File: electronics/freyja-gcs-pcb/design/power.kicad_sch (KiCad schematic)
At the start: 122 parts, among them J6 GT-USB-7010ASV, J7 A2543WR-4P-2, J8 XD-PH-10AW, J9 JS350-S02DCA-00, Q1 TM10N06SI, Q2 TM10N06SI, Q3 AO4459, Q4 L2N7002SLLT1G, Q5 L2N7002SLLT1G, Q6 TM10N06SI, Q7 TM10N06SI, Q8 TM10N06SI, SW3 K6-6136D-L1-04, U10 LM74700QDBVRQ1, U11 AMS1117-3.3, U12 RY3730, U3 FM7021DB, U4 CN3702, U5 HY2213-BB3A, U6 HY2213-BB3A, U7 IP2721, U8 SY8368AQQC, U9 LM74700QDBVRQ1

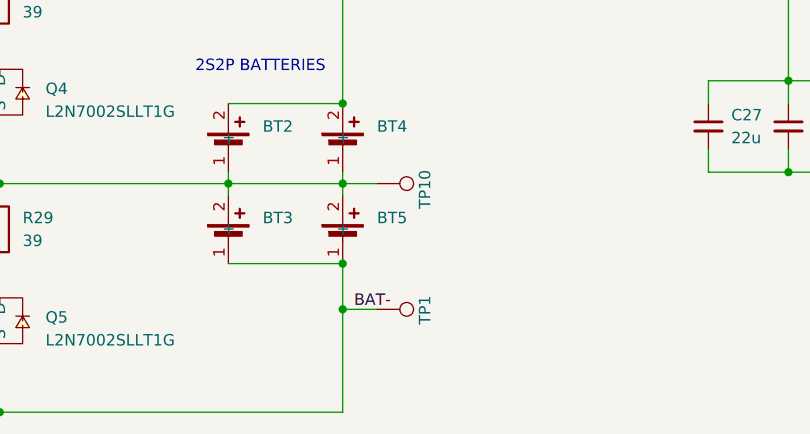
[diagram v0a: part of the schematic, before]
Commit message: cleanup
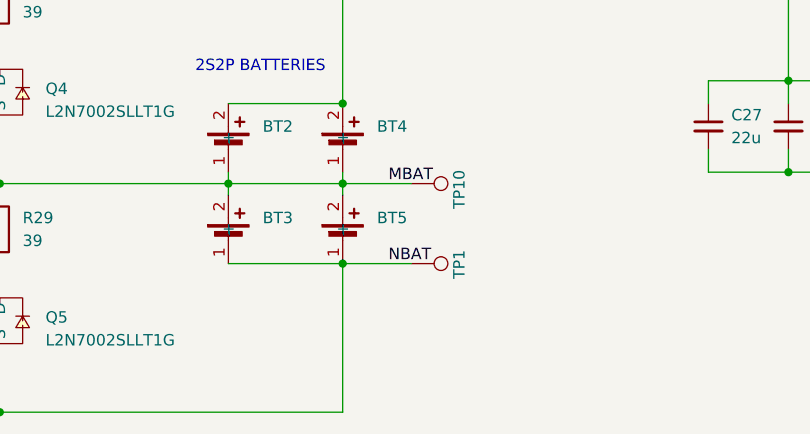
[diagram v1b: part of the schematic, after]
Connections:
- net MBAT: now reaches BT2.1 (-), BT3.2 (+), BT4.1 (-), BT5.2 (+), C21.2, Q4.2 (S), R22.2, R24.1, R29.1, TP10.1, U5.3 (VSS)
- net BAT- renamed NBAT
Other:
- moved on the sheet: TP1, TP10
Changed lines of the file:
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@@
 	)
 	(junction
-		(at 170.18 246.38)
-		(diameter 0)
-		(color 0 0 0 0)
-	)
-	(junction
 		(at 303.53 146.05)
 		(diameter 0)
@@
 	(wire
 		(pts
-			(xy 170.18 246.38) (xy 170.18 257.81)
-		)
-		(stroke
-			(width 0)
-			(type default)
-		)
-	)
-	(wire
-		(pts
 			(xy 274.32 175.26) (xy 276.86 175.26)
 		)
@@
 	(wire
 		(pts
-			(xy 170.18 241.3) (xy 170.18 246.38)
-		)
-		(stroke
-			(width 0)
-			(type default)
-		)
-	)
-	(wire
-		(pts
 			(xy 148.59 44.45) (xy 148.59 49.53)
 		)
@@
 	(wire
 		(pts
+			(xy 170.18 241.3) (xy 170.18 257.81)
+		)
+		(stroke
+			(width 0)
+			(type default)
+		)
+	)
+	(wire
+		(pts
 			(xy 85.09 132.08) (xy 85.09 134.62)
 		)
@@
 	(wire
 		(pts
-			(xy 170.18 246.38) (xy 173.99 246.38)
+			(xy 170.18 241.3) (xy 177.8 241.3)
 		)
 		(stroke
@@
 	(wire
 		(pts
-			(xy 170.18 232.41) (xy 173.99 232.41)
+			(xy 170.18 232.41) (xy 177.8 232.41)
 		)
 		(stroke
@@
 		)
 	)
-	(label "BAT-"
-		(at 171.45 246.38 0)
+	(label "NBAT"
+		(at 175.26 241.3 0)
+		(effects
+			(font
+				(size 1.27 1.27)
+			)
+			(justify left bottom)
+		)
+	)
+	(label "MBAT"
+		(at 175.26 232.41 0)
 		(effects
 			(font
@@
 	(symbol
 		(lib_id "Connector:TestPoint")
-		(at 173.99 232.41 270)
+		(at 177.8 232.41 270)
 		(unit 1)
 		(exclude_from_sim no)
@@
 		(dnp no)
 		(property "Reference" "TP10"
-			(at 179.324 230.886 0)
+			(at 183.134 230.886 0)
 			(effects
 				(font
@@
 		)
 		(property "Value" "TestPoint"
-			(at 176.0221 234.95 0)
+			(at 179.8321 234.95 0)
 			(effects
 				(font
@@
 		)
 		(property "Footprint" "TestPoint:TestPoint_Pad_D3.0mm"
-			(at 173.99 237.49 0)
+			(at 177.8 237.49 0)
 			(effects
 				(font
@@
 		)
 		(property "Datasheet" "~"
-			(at 173.99 237.49 0)
+			(at 177.8 237.49 0)
 			(effects
 				(font
@@
 		)
 		(property "Description" "test point"
-			(at 173.99 232.41 0)
+			(at 177.8 232.41 0)
 			(effects
 				(font
@@
 	(symbol
 		(lib_id "Connector:TestPoint")
-		(at 173.99 246.38 270)
+		(at 177.8 241.3 270)
 		(unit 1)
 		(exclude_from_sim no)
@@
 		(dnp no)
 		(property "Reference" "TP1"
-			(at 179.324 244.856 0)
+			(at 183.134 239.776 0)
 			(effects
 				(font
@@
 		)
 		(property "Value" "TestPoint"
-			(at 176.0221 248.92 0)
+			(at 179.8321 243.84 0)
 			(effects
 				(font
@@
 		)
 		(property "Footprint" "TestPoint:TestPoint_Pad_D3.0mm"
-			(at 173.99 251.46 0)
+			(at 177.8 246.38 0)
 			(effects
 				(font
@@
 		)
 		(property "Datasheet" "~"
-			(at 173.99 251.46 0)
+			(at 177.8 246.38 0)
 			(effects
 				(font
@@
 		)
 		(property "Description" "test point"
-			(at 173.99 246.38 0)
+			(at 177.8 241.3 0)
 			(effects
 				(font
